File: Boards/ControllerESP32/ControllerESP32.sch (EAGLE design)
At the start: 10 parts

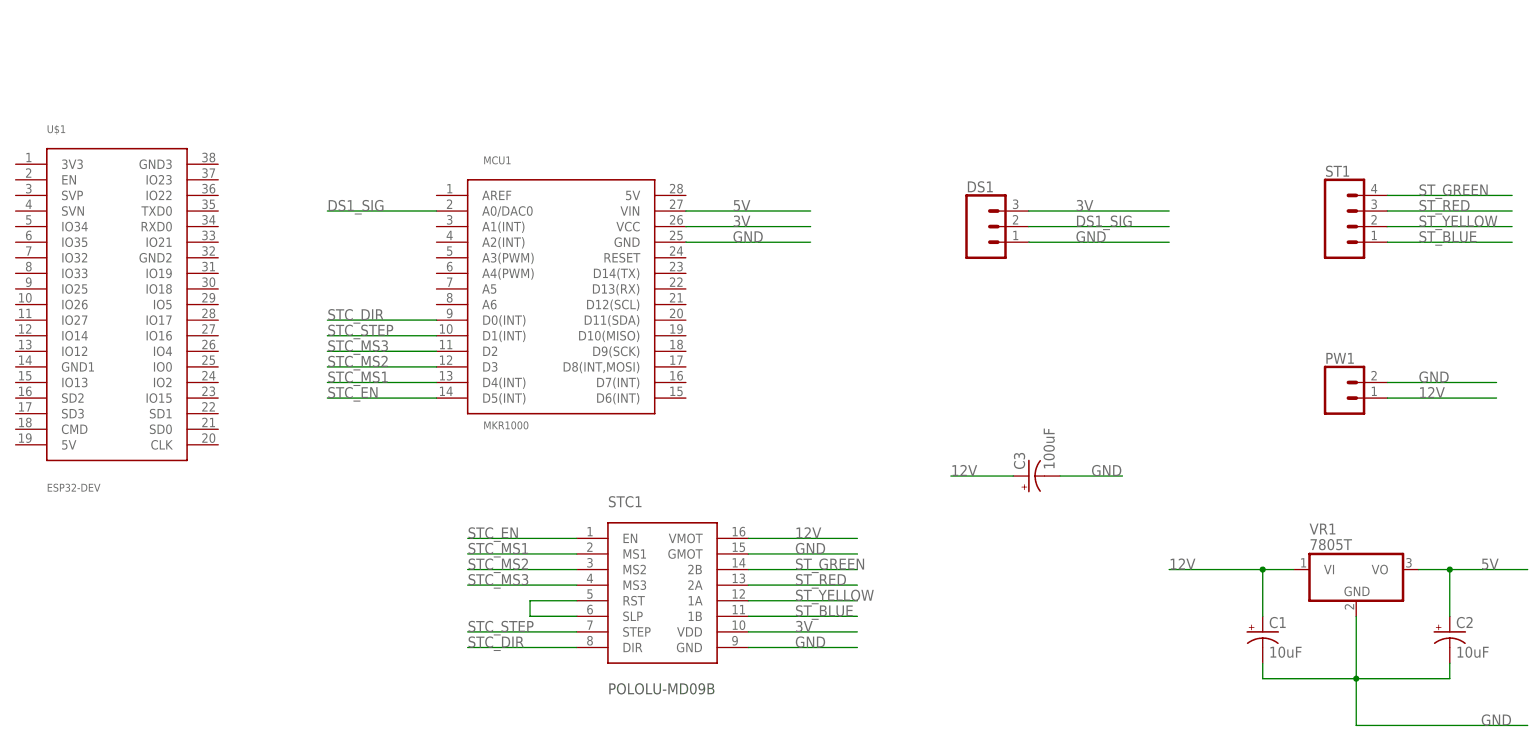
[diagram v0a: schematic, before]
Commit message: finished esp32 based board
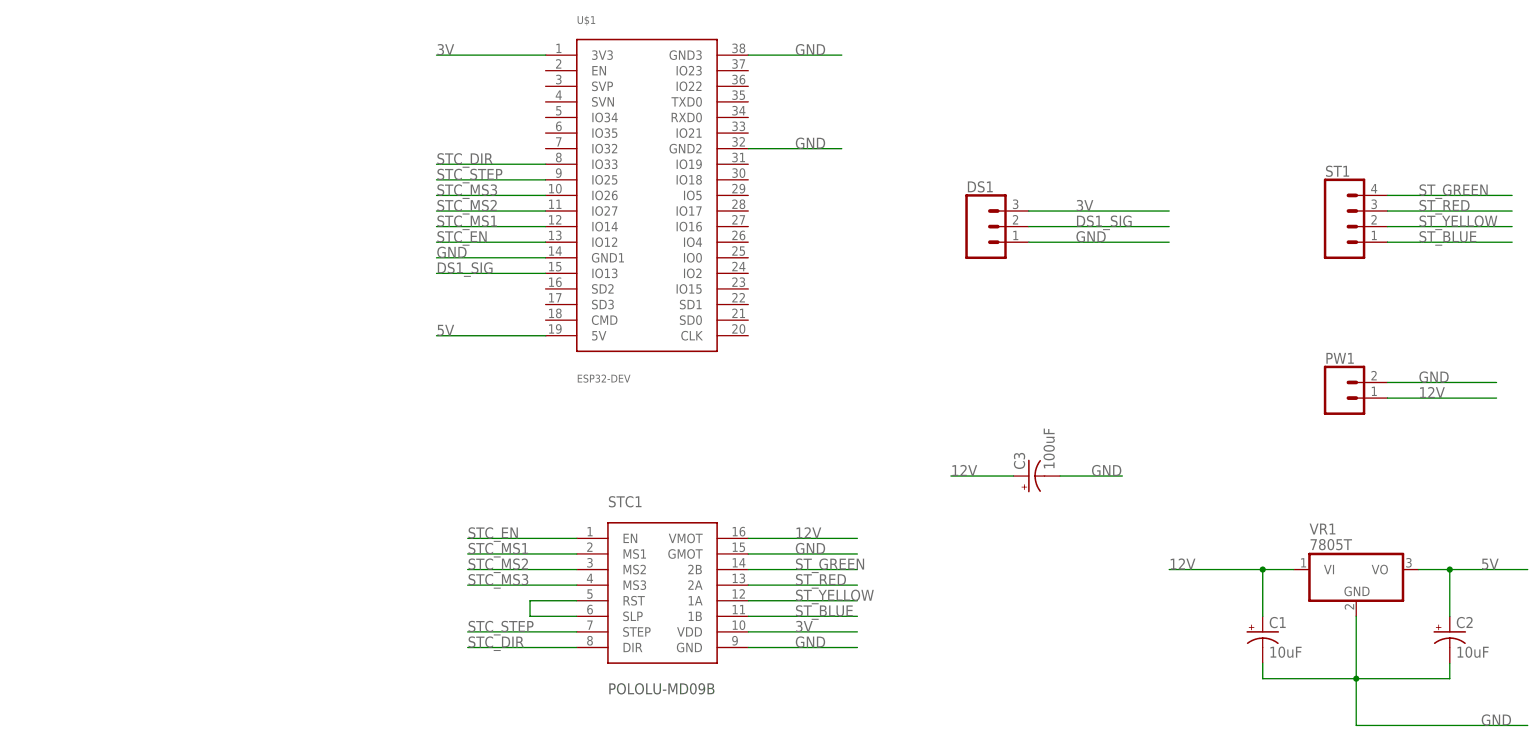
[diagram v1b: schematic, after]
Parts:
- removed MCU1: MKR1000, Library:MKR1000
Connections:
- net 3V: now also U$1.3V3; no longer MCU1.VCC
- net 5V: now also U$1.5V; no longer MCU1.VIN
- net DS1_SIG: now also U$1.IO13; no longer MCU1.A0/DAC0
- net GND: now also U$1.GND1, U$1.GND2, U$1.GND3; no longer MCU1.GND
- net STC_DIR: now also U$1.IO33; no longer MCU1.D0(INT)
- net STC_EN: now also U$1.IO12; no longer MCU1.D5(INT)
- net STC_MS1: now also U$1.IO14; no longer MCU1.D4(INT)
- net STC_MS2: now also U$1.IO27; no longer MCU1.D3
- net STC_MS3: now also U$1.IO26; no longer MCU1.D2
- net STC_STEP: now also U$1.IO25; no longer MCU1.D1(INT)
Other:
- moved on the sheet: U$1
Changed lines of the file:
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@@
 </classes>
 <parts>
-<part name="MCU1" library="Library" deviceset="MKR1000" device=""/>
 <part name="STC1" library="Library" deviceset="POLOLU-MD09B" device=""/>
 <part name="PW1" library="SparkFun-Connectors" deviceset="CONN_02" device="5MM"/>
@@
 </plain>
 <instances>
-<instance part="MCU1" gate="G$1" x="30.48" y="60.96"/>
 <instance part="STC1" gate="G$1" x="48.26" y="12.7"/>
 <instance part="PW1" gate="G$1" x="157.48" y="45.72"/>
@@
 <instance part="C3" gate="G$1" x="106.68" y="33.02" rot="R90"/>
 <instance part="DS1" gate="J$1" x="99.06" y="73.66"/>
-<instance part="U$1" gate="G$1" x="-43.18" y="60.96"/>
+<instance part="U$1" gate="G$1" x="43.18" y="78.74"/>
 </instances>
 <busses>
@@
 <nets>
 <net name="GND" class="0">
-<segment>
-<pinref part="MCU1" gate="G$1" pin="GND"/>
-<wire x1="50.8" y1="71.12" x2="71.12" y2="71.12" width="0.1524" layer="91"/>
-<label x="58.42" y="71.12" size="1.778" layer="95"/>
-</segment>
 <segment>
 <pinref part="STC1" gate="G$1" pin="GND"/>
@@
 <label x="114.3" y="71.12" size="1.778" layer="95"/>
 </segment>
+<segment>
+<pinref part="U$1" gate="G$1" pin="GND3"/>
+<wire x1="60.96" y1="101.6" x2="76.2" y2="101.6" width="0.1524" layer="91"/>
+<label x="68.58" y="101.6" size="1.778" layer="95"/>
+</segment>
+<segment>
+<pinref part="U$1" gate="G$1" pin="GND2"/>
+<wire x1="60.96" y1="86.36" x2="76.2" y2="86.36" width="0.1524" layer="91"/>
+<label x="68.58" y="86.36" size="1.778" layer="95"/>
+</segment>
+<segment>
+<pinref part="U$1" gate="G$1" pin="GND1"/>
+<wire x1="27.94" y1="68.58" x2="10.16" y2="68.58" width="0.1524" layer="91"/>
+<label x="10.16" y="68.58" size="1.778" layer="95"/>
+</segment>
 </net>
 <net name="3V" class="0">
-<segment>
-<pinref part="MCU1" gate="G$1" pin="VCC"/>
-<wire x1="50.8" y1="73.66" x2="71.12" y2="73.66" width="0.1524" layer="91"/>
-<label x="58.42" y="73.66" size="1.778" layer="95"/>
-</segment>
 <segment>
 <pinref part="STC1" gate="G$1" pin="VDD"/>
@@
 <wire x1="106.68" y1="76.2" x2="129.54" y2="76.2" width="0.1524" layer="91"/>
 <label x="114.3" y="76.2" size="1.778" layer="95"/>
+</segment>
+<segment>
+<pinref part="U$1" gate="G$1" pin="3V3"/>
+<wire x1="27.94" y1="101.6" x2="10.16" y2="101.6" width="0.1524" layer="91"/>
+<label x="10.16" y="101.6" size="1.778" layer="95"/>
 </segment>
 </net>
@@
 </segment>
 <segment>
-<pinref part="MCU1" gate="G$1" pin="D5(INT)"/>
-<wire x1="10.16" y1="45.72" x2="-7.62" y2="45.72" width="0.1524" layer="91"/>
-<label x="-7.62" y="45.72" size="1.778" layer="95"/>
+<pinref part="U$1" gate="G$1" pin="IO12"/>
+<wire x1="27.94" y1="71.12" x2="10.16" y2="71.12" width="0.1524" layer="91"/>
+<label x="10.16" y="71.12" size="1.778" layer="95"/>
 </segment>
 </net>
@@
 </segment>
 <segment>
-<pinref part="MCU1" gate="G$1" pin="D0(INT)"/>
-<wire x1="10.16" y1="58.42" x2="-7.62" y2="58.42" width="0.1524" layer="91"/>
-<label x="-7.62" y="58.42" size="1.778" layer="95"/>
+<pinref part="U$1" gate="G$1" pin="IO33"/>
+<wire x1="27.94" y1="83.82" x2="10.16" y2="83.82" width="0.1524" layer="91"/>
+<label x="10.16" y="83.82" size="1.778" layer="95"/>
 </segment>
 </net>
@@
 </segment>
 <segment>
-<pinref part="MCU1" gate="G$1" pin="D1(INT)"/>
-<wire x1="10.16" y1="55.88" x2="-7.62" y2="55.88" width="0.1524" layer="91"/>
-<label x="-7.62" y="55.88" size="1.778" layer="95"/>
+<pinref part="U$1" gate="G$1" pin="IO25"/>
+<wire x1="27.94" y1="81.28" x2="10.16" y2="81.28" width="0.1524" layer="91"/>
+<label x="10.16" y="81.28" size="1.778" layer="95"/>
 </segment>
 </net>
@@
 </segment>
 <segment>
-<pinref part="MCU1" gate="G$1" pin="D2"/>
-<wire x1="10.16" y1="53.34" x2="-7.62" y2="53.34" width="0.1524" layer="91"/>
-<label x="-7.62" y="53.34" size="1.778" layer="95"/>
+<pinref part="U$1" gate="G$1" pin="IO26"/>
+<wire x1="27.94" y1="78.74" x2="10.16" y2="78.74" width="0.1524" layer="91"/>
+<label x="10.16" y="78.74" size="1.778" layer="95"/>
 </segment>
 </net>
@@
 </segment>
 <segment>
-<pinref part="MCU1" gate="G$1" pin="D4(INT)"/>
-<wire x1="10.16" y1="48.26" x2="-7.62" y2="48.26" width="0.1524" layer="91"/>
-<label x="-7.62" y="48.26" size="1.778" layer="95"/>
+<pinref part="U$1" gate="G$1" pin="IO14"/>
+<wire x1="27.94" y1="73.66" x2="10.16" y2="73.66" width="0.1524" layer="91"/>
+<label x="10.16" y="73.66" size="1.778" layer="95"/>
 </segment>
 </net>
@@
 </segment>
 <segment>
-<pinref part="MCU1" gate="G$1" pin="D3"/>
-<wire x1="10.16" y1="50.8" x2="-7.62" y2="50.8" width="0.1524" layer="91"/>
-<label x="-7.62" y="50.8" size="1.778" layer="95"/>
+<pinref part="U$1" gate="G$1" pin="IO27"/>
+<wire x1="27.94" y1="76.2" x2="10.16" y2="76.2" width="0.1524" layer="91"/>
+<label x="10.16" y="76.2" size="1.778" layer="95"/>
 </segment>
 </net>
@@
 </segment>
 <segment>
-<pinref part="MCU1" gate="G$1" pin="VIN"/>
-<wire x1="50.8" y1="76.2" x2="71.12" y2="76.2" width="0.1524" layer="91"/>
-<label x="58.42" y="76.2" size="1.778" layer="95"/>
+<pinref part="U$1" gate="G$1" pin="5V"/>
+<wire x1="27.94" y1="55.88" x2="10.16" y2="55.88" width="0.1524" layer="91"/>
+<label x="10.16" y="55.88" size="1.778" layer="95"/>
 </segment>
 </net>
@@
 </segment>
 <segment>
-<pinref part="MCU1" gate="G$1" pin="A0/DAC0"/>
-<wire x1="10.16" y1="76.2" x2="-7.62" y2="76.2" width="0.1524" layer="91"/>
-<label x="-7.62" y="76.2" size="1.778" layer="95"/>
-</segment>
-</net>
+<pinref part="U$1" gate="G$1" pin="IO13"/>
+<wire x1="27.94" y1="66.04" x2="10.16" y2="66.04" width="0.1524" layer="91"/>
+<label x="10.16" y="66.04" size="1.778" layer="95"/>
+</segment>
+</net>
